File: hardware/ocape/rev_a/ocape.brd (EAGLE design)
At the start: 54.6 x 59.9 mm, 12 parts, among them J1 CON_HEADER_2X05-PTH+SHROUDED_A, J2 JUMPER-PTH-2-NO, P9/P8 BBB_HEADERS, U1 CAT24C256WI-GT3

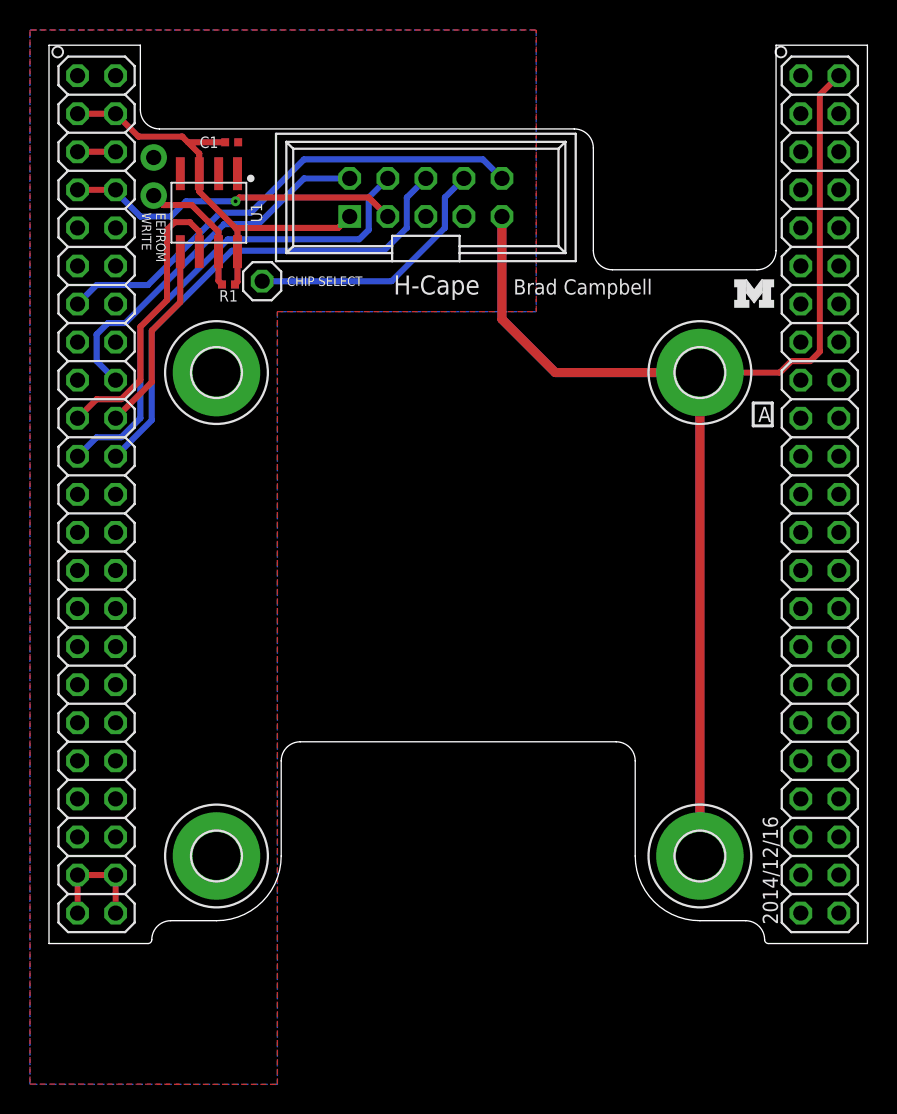
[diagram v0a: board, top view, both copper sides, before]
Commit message: shipped rev a
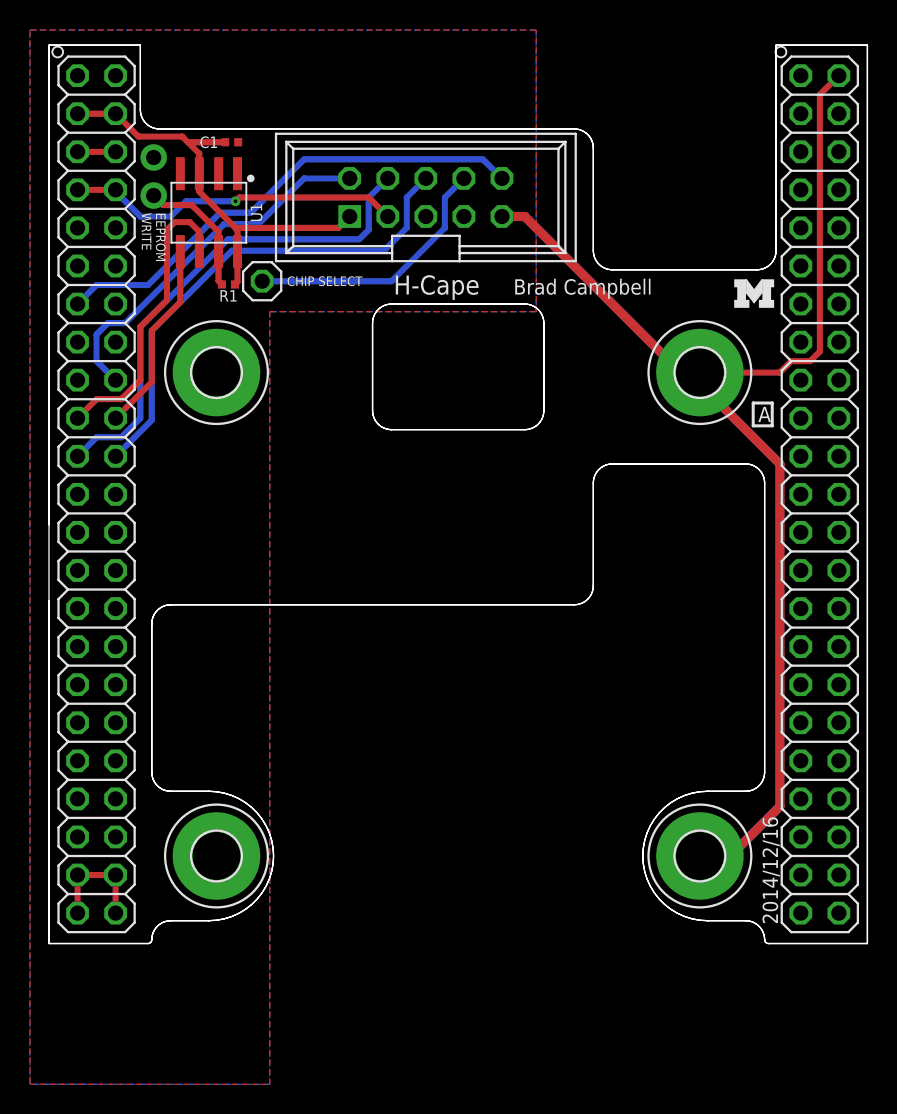
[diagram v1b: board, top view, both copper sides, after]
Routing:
- net GND: track 142.7 -> 145.9 mm
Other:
- outline, holes or cut-outs redrawn
- board text removed: "CE1"
